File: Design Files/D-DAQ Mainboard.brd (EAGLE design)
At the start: 99.8 x 49.9 mm, 121 parts, among them Y1 XTC7009, Y2 DS1099

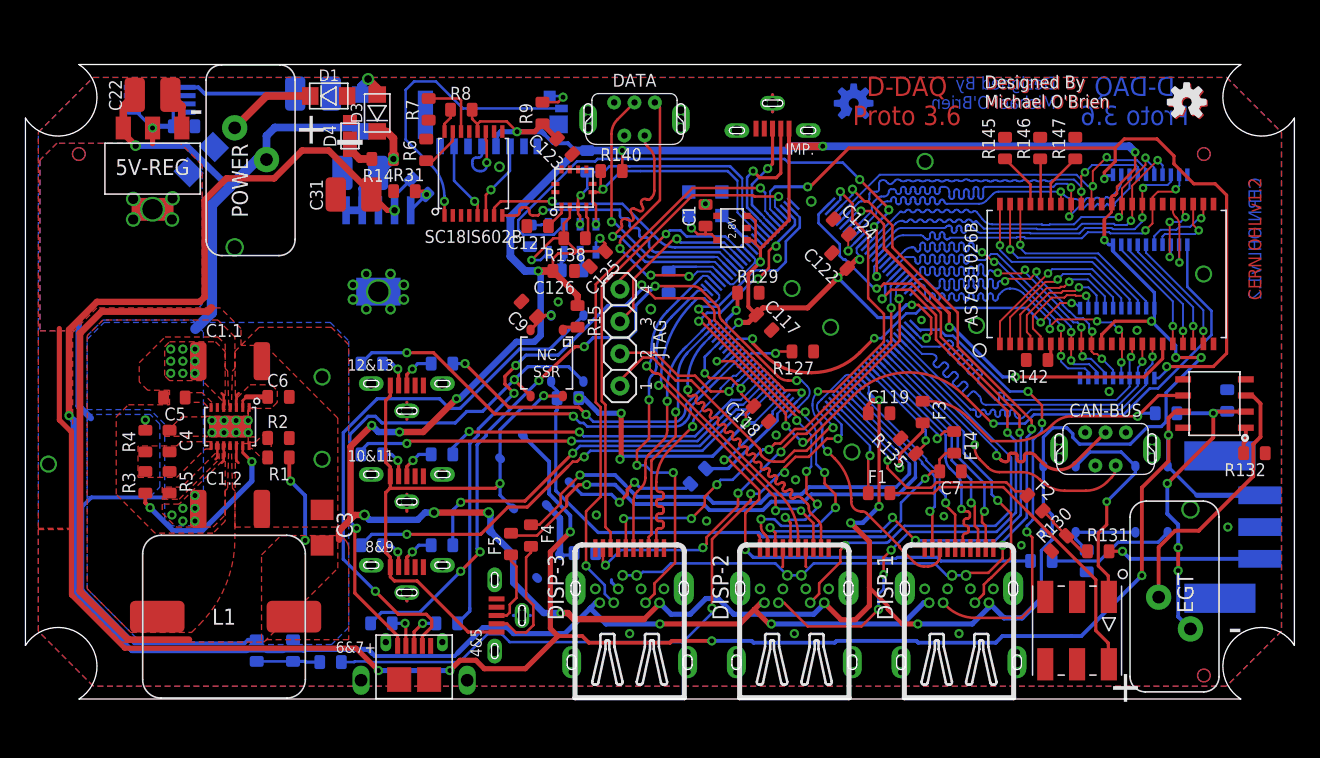
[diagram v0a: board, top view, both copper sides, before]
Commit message: Updating to Proto 4
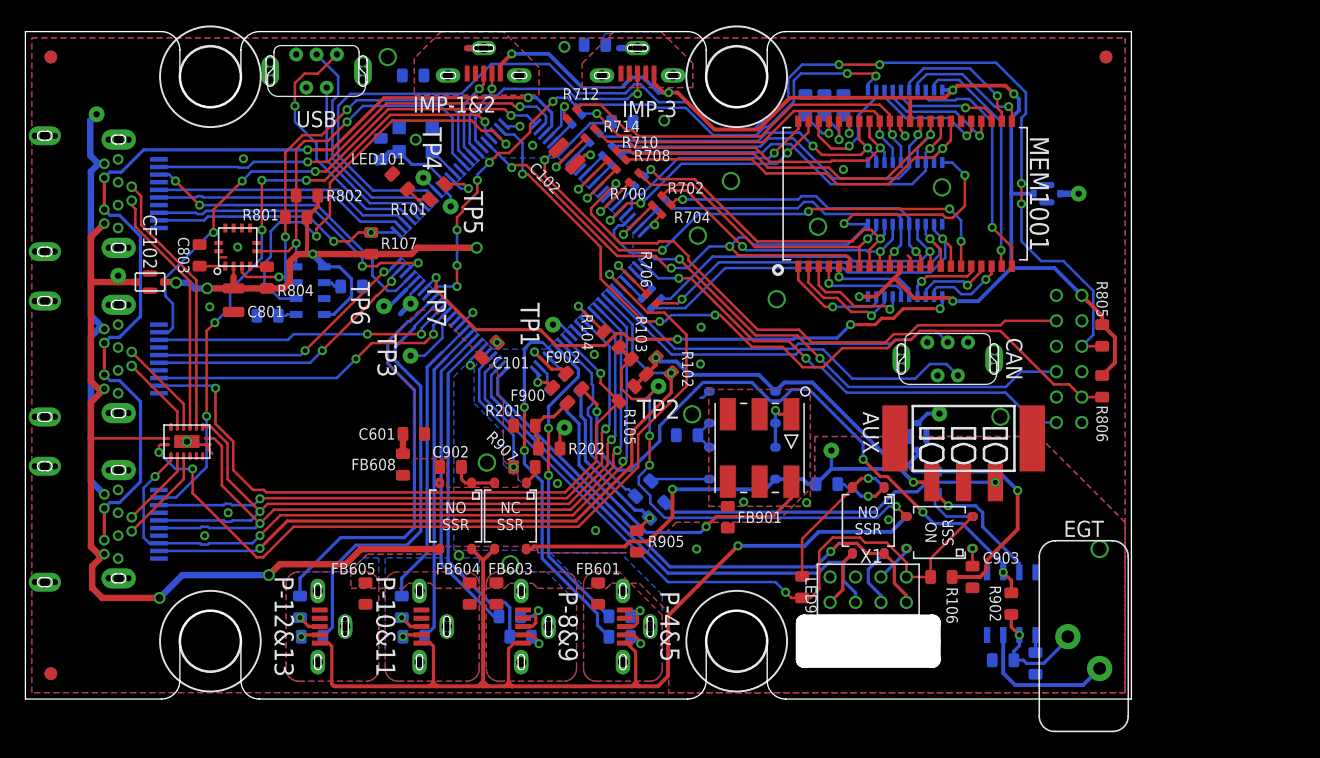
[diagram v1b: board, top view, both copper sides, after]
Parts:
- removed 10&11, 12&13, 4&5, 8&9, IMP.: Micro USB, Parts for D-DAQ:USB-MICRO-B-VERT
- removed 14V-REG: TL1963A-33DCQ, Parts for D-DAQ:SOT-223-6
- removed 2.8V: TC1016-2.8VCTTR, Parts for D-DAQ:SOT-23-5
- removed 3.3V-TOGGLE-1, 3.3V-TOGGLE-2, 3.3V-TOGGLE-3: NO SSR, Parts for D-DAQ:SOP-4-NO
- removed 5V-REG: ZLDO1117-5.0, Parts for D-DAQ:SOT-223-4
- removed 5V-TOGGLE-1, 5V-TOGGLE-2, 5V-TOGGLE-3: NC SSR, Parts for D-DAQ:SOP-4-NC
- removed 6&7+: Micro USB, Parts for D-DAQ:USB-MICRO-AB-FLAT
- removed AS7C31026B: 1 Mbit SRAM, Parts for D-DAQ:TSOP-44
- removed AUX-PRESS: PC-1771101, Parts for D-DAQ:PC-1771101
- removed C1, C6: 10nF, Parts for D-DAQ:SMD-0603
- removed C1.1, C1.2: 22uF, Parts for D-DAQ:SMD-1812-EDGE
- removed C10, C11, C123, C9: 4.7uF, Parts for D-DAQ:SMD-0603
- removed C117, C118, C119, C121, C122, C126, C127, C5, C7, C8: 0.1uF, Parts for D-DAQ:SMD-0603
- removed C124, C125, C2: 22uF, Parts for D-DAQ:SMD-0603
- removed C2.1, C2.2, C22, C31: 10uF, Parts for D-DAQ:SMD-1210
- removed C21: 4.7uF, Parts for D-DAQ:SMD-1206
- removed C3: 47uF, Parts for D-DAQ:SMD-1206
- removed C4: 1uF, Parts for D-DAQ:SMD-0603
- removed CAN-BUS, DATA: UE25BE5510H, Parts for D-DAQ:USB-MINI-B-VERT
- removed D1: S07D-GS08, Parts for D-DAQ:DO-219AB-2
- removed D2, D3: PMEG2010ER, Parts for D-DAQ:DO-219AB-2
- removed D4: TFZGTR20B, Parts for D-DAQ:TUMD2
- removed EGT-AMP: MAX4239, Parts for D-DAQ:SOT-8
- removed F0, F1, F10, F11, F12, F13, F14, F2, F3, F4, F5, F6, F7, F8, F9: 470, Parts for D-DAQ:SMD-0603
- removed JTAG: HEADER-X4, Parts for D-DAQ:HEADER-X4
- removed L1: 7.6uH, Parts for D-DAQ:7443551XXX
- removed LATCH-HIGH, LATCH-LOW: Octal D-Latch, Parts for D-DAQ:TSSOP-20
- removed MAIN-SMPS: MP2209, Parts for D-DAQ:QFN-14
- removed MICRO-SD: 47579-0001, Parts for D-DAQ:SCHA4B0400
- removed MMA8652FC: Accelerometer, Parts for D-DAQ:QFN-12
- removed MPL3115A101: Baro & Temp, Parts for D-DAQ:LGA-8
- removed NBPLANN100PAUNV: Boost, Parts for D-DAQ:LEADLESS-SMT
- removed PIC32MX: 795F512L-80V/PT, Parts for D-DAQ:TQFP-100-12X12
- removed POWER: 1702610, Parts for D-DAQ:PC-1702610
- removed R1: 499k, Parts for D-DAQ:SMD-0603
- removed R10, R12, R127, R129, R130, R132, R135, R138, R139, R142, R145, R146, R147, R6, R7, R8, R9: 10k, Parts for D-DAQ:SMD-0603
- removed R11, R136, R140, R141: 1.4k, Parts for D-DAQ:SMD-0603
- removed R131: 255, Parts for D-DAQ:SMD-0603
- removed R133, R3, R5: 100k, Parts for D-DAQ:SMD-0603
- removed R14: 33.2, Parts for D-DAQ:SMD-0603
- removed R15, R20, R21: 100, Parts for D-DAQ:SMD-0603
- removed R2: 158k, Parts for D-DAQ:SMD-0603
- removed R31: 3.01k, Parts for D-DAQ:SMD-0603
- removed R32: 30.9k, Parts for D-DAQ:SMD-0603
- removed R4: 10, Parts for D-DAQ:SMD-0603
- removed SC18IS602B: I2C to SPI, Parts for D-DAQ:TSSOP-16
- removed U$6, U$7: (no value), Parts for D-DAQ:OSHW-LOGO-S
- removed Y1: XTC7009, Parts for D-DAQ:3.2X2.5MM
- removed Y2: DS1099, Parts for D-DAQ:SOIC-8
- added 12V, 14V, 3.3V, 3.3V-2, 3.3V-3, 5V, TP1, TP2, TP3, TP4, TP5, TP6, TP7: TP-0463, Parts for D-DAQ:TP-REC
- added AUX: PC-3-1771101, Parts for D-DAQ:PC-1771101
- added BFID-1, BFID-2, BFID-3, TFID-1, TFID-2, TFID-3: (no value), Parts for D-DAQ:1MM-FIDUCIAL
- added C101, C601, C802, C803: 0.1uF, Parts for D-DAQ:SMD-0603
- added C102, C801: 10uF, Parts for D-DAQ:SMD-0805
- added C103: 10nF, Parts for D-DAQ:SMD-0603
- added C901, C902, C903: 4.7uF, Parts for D-DAQ:SMD-0603
- added CAN, USB: UE25BE5510H, Parts for D-DAQ:USB-MINI-B-VERT
- added CF101, CF102, CF103: (no value), Parts for D-DAQ:NFM21PS
- added F900, F901, F902, F903, F904, F905, F908, F909, F910, F911, F912, F913, FB601, FB603, FB604, FB605, FB606, FB607, FB608, FB901, R104: 470, Parts for D-DAQ:SMD-0603
- added HOLE-BL, HOLE-BR, HOLE-ML, HOLE-MR: (no value), Parts for D-DAQ:3.2-GRMT
- added IMP-1&2, IMP-3, P-10&11, P-12&13, P-4&5, P-8&9: Micro USB, Parts for D-DAQ:USB-MICRO-B-VERT
- added K1001, K1003, K1005: NC SSR, Parts for D-DAQ:SOP-4-NC
- added K1002, K1004, K1006, K1007, K1008: NO SSR, Parts for D-DAQ:SOP-4-NO
- added LED101: Yellow, Parts for D-DAQ:SMD-0603
- added LED901: Red, Parts for D-DAQ:SMD-0603
- added MEM1001: IS61WV25616ALL, Parts for D-DAQ:TSOP-44
- added OSHW-BOT, OSHW-TOP: (no value), Parts for D-DAQ:OSHW-LOGO-L
- added R101, R102, R103, R105, R106, R107, R202, R716, R717, R718, R719, R803, R804, R805, R806, R903, R905: 10k, Parts for D-DAQ:SMD-0603
- added R201, R801, R802, R901: 1.4k, Parts for D-DAQ:SMD-0603
- added R700, R701, R702, R703, R704, R705, R706, R707, R708, R709, R710, R711, R712, R713, R714, R715: 140, Parts for D-DAQ:SMD-0402
- added R902: 100k, Parts for D-DAQ:SMD-0603
- added R904: 255, Parts for D-DAQ:SMD-0603
- added R906, R907, R908, R909: 100, Parts for D-DAQ:SMD-0603
- added U1001: 795F512L-80V/PT, Parts for D-DAQ:TQFP-100-14X14
- added U1002, U1003: Octal D-Latch, Parts for D-DAQ:TSSOP-20
- added U1004: Baro & Temp, Parts for D-DAQ:LGA-8
- added U1005: Boost, Parts for D-DAQ:LEADLESS-SMT
- added U1006: Accelerometer, Parts for D-DAQ:QFN-12
- added U1007: MAX4239, Parts for D-DAQ:SOT-8
- added U1008: NXP-74HC165, Parts for D-DAQ:DHVQFN16
- added X1: (no value), Parts for D-DAQ:MOLEX-87760-0816
- added X3: MOLEX-87760-1216", Parts for D-DAQ:MOLEX-87760-1216
- added Y1001: XTC7009, Parts for D-DAQ:3.2X2.5MM
- EGT: value 1702610 -> (none)
- moved DISP-1 77.1 mm to (4.25, 39.8), flipped to the bottom, turned to 90 degrees
- moved DISP-2 60.1 mm to (4.25, 26.8), flipped to the bottom, turned to 90 degrees
- moved DISP-3 44.0 mm to (4.25, 13.8), flipped to the bottom, turned to 90 degrees
- moved EGT 7.79 mm to (83.2, 3.65)
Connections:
- removed net 100-PSI-SENSOR-RES: 5V-TOGGLE-2.1, R20.2
- removed net 12V-BS: C5.1, MAIN-SMPS.7
- removed net 12V-ENABLE: MAIN-SMPS.13, R3.1
- removed net 12V-FB: MAIN-SMPS.P14, R1.2, R2.1
- removed net 12V-OK: MAIN-SMPS.9, R5.2
- removed net 12V-SS: C6.1, MAIN-SMPS.2
- removed net 12V-SW: C5.2, L1.P$1, MAIN-SMPS.11, MAIN-SMPS.4
- removed net 12V-VCC: C4.2, MAIN-SMPS.8, R3.2, R4.1, R5.1
- removed net 14V-12V-DIVIDER: F0.2, R10.2, R11.2
- removed net 14V-ADJ: 14V-REG.ADJ, R31.2, R32.1
- removed net 14V-INPUT: 14V-REG.SHDN, 14V-REG.VIN, C2.2.1, D3.P$2, R14.1
- removed net 3.3-&-5V-TOGGLE1: PIC32MX.28, R21.1
- removed net 3.3-&-5V-TOGGLE2: PIC32MX.29, R20.1
- removed net 3.3V-RAIL: 2.8V.1, 2.8V.3, 3.3V-TOGGLE-1.3, 3.3V-TOGGLE-2.3, AS7C31026B.11, AS7C31026B.33, C117.1, C118.2, C119.1, C122.1, C123.2, C125.1, C126.2, C2.2, C3.2, DISP-1.4, DISP-2.4, DISP-3.4, IMP..1, L1.P$2, LATCH-HIGH.20, LATCH-LOW.20, MICRO-SD.4, MMA8652FC.2, MPL3115A101.1, MPL3115A101.4, PIC32MX.16, PIC32MX.2, PIC32MX.30, PIC32MX.37, PIC32MX.46, PIC32MX.55, PIC32MX.62, PIC32MX.86, R1.1, R12.1, R138.2, R140.2, R141.1, R15.1, R8.2, R9.1, SC18IS602B.12
- removed net 5V-ADJ: 5V-REG.ADJ, C22.2
- removed net 6&7-PIN1: 3.3V-TOGGLE-3.3, 5V-TOGGLE-3.3, 6&7+.1
- removed net A0-PD: R7.2, SC18IS602B.14
- removed net A1-PD: R6.1, SC18IS602B.15
- removed net A2-PU: R8.1, SC18IS602B.16
- removed net ADD-0: AS7C31026B.5, LATCH-LOW.12
- removed net ADD-1: AS7C31026B.4, LATCH-LOW.13
- removed net ADD-10: AS7C31026B.25, LATCH-HIGH.14
- removed net ADD-11: AS7C31026B.24, LATCH-HIGH.15
- removed net ADD-12: AS7C31026B.21, LATCH-HIGH.16
- removed net ADD-13: AS7C31026B.20, LATCH-HIGH.17
- removed net ADD-14: AS7C31026B.19, LATCH-HIGH.18
- removed net ADD-15: AS7C31026B.18, LATCH-HIGH.19
- removed net ADD-2: AS7C31026B.3, LATCH-LOW.14
- removed net ADD-3: AS7C31026B.2, LATCH-LOW.15
- removed net ADD-4: AS7C31026B.1, LATCH-LOW.16
- removed net ADD-5: AS7C31026B.44, LATCH-LOW.17
- removed net ADD-6: AS7C31026B.43, LATCH-LOW.18
- removed net ADD-7: AS7C31026B.42, LATCH-LOW.19
- removed net ADD-8: AS7C31026B.27, LATCH-HIGH.12
- removed net ADD-9: AS7C31026B.26, LATCH-HIGH.13
- removed net AN2-OIL-PESS: F2.1, PIC32MX.23
- removed net AN3-EGT: F3.2, PIC32MX.22
- removed net AN6: 6&7+.2, F6.1
- removed net AN7: 6&7+.3, F7.2
- removed net AUTO-DETECT: 5V-TOGGLE-1.1, R21.2
- removed net BARO-INT2: MPL3115A101.5, R139.1
- removed net CAN-BUS1: CAN-BUS.2, PIC32MX.8
- removed net CAN-BUS2: CAN-BUS.3, PIC32MX.7
- removed net CARD-DETECT: MICRO-SD.G3, SC18IS602B.1
- removed net CE: AS7C31026B.6, R142.1
- removed net CHARG-CAPS: C2.1.1, Y2.1
- removed net CP-PUMP: C2.1.2, D2.P$2, D3.P$1
- removed net CPS-INPUT: IMP..2, PIC32MX.68
- removed net CRYSTAL-OUT: PIC32MX.63
- removed net DISP-1_HPD: DISP-1.6, PIC32MX.9
- removed net DISP-HPD2: DISP-2.6, PIC32MX.6
- removed net DISP-HPD3: DISP-3.6, PIC32MX.51
- removed net EGT-SHTDWN: EGT-AMP.1, R132.2
- removed net GND: 10&11.5, 10&11.T0, 10&11.T1, 10&11.T2, 12&13.5, 12&13.T0, 12&13.T1, 12&13.T2, 14V-REG.GND, 14V-REG.TAB, 2.8V.2, 3.3V-TOGGLE-1.2, 3.3V-TOGGLE-2.2, 4&5.5, 4&5.T0, 4&5.T1, 4&5.T2, 6&7+.5, 6&7+.B1, 6&7+.B2, 6&7+.F1, 6&7+.F2, 8&9.5, 8&9.T0, 8&9.T1, 8&9.T2, AS7C31026B.12, AS7C31026B.34, AUX-PRESS.P2, AUX-PRESS.T0, AUX-PRESS.T1, C1.1.2, C1.2, C1.2.2, C10.1, C11.1, C117.2, C118.1, C119.2, C121.2, C122.2, C123.1, C124.1, C125.2, C126.1, C127.1, C2.1, C2.2.2, C21.2, C3.1, C31.1, C4.1, C6.2, C7.1, C8.2, C9.2, CAN-BUS.5, CAN-BUS.P$1, CAN-BUS.P$2, CAN-BUS.P$3, CAN-BUS.P$4, CAN-BUS.T0, CAN-BUS.T1, D1.P$1, D4.P$1, DATA.5, DATA.P$1, DATA.P$2, DATA.P$3, DATA.P$4, DATA.T0, DATA.T1, DISP-1.1, DISP-1.13, DISP-1.14, DISP-1.19, DISP-1.7, DISP-1.8, DISP-1.BL, DISP-1.BR, DISP-1.FL, DISP-1.FR, DISP-2.1, DISP-2.13, DISP-2.14, DISP-2.19, DISP-2.7, DISP-2.8, DISP-2.BL, DISP-2.BR, DISP-2.FL, DISP-2.FR, DISP-3.1, DISP-3.13, DISP-3.14, DISP-3.19, DISP-3.7, DISP-3.8, DISP-3.BL, DISP-3.BR, DISP-3.FL, DISP-3.FR, EGT-AMP.4, IMP..5, IMP..T0, IMP..T1, IMP..T2, LATCH-HIGH.10, LATCH-LOW.10, MAIN-SMPS.1, MAIN-SMPS.12, MAIN-SMPS.3, MAIN-SMPS.P$15, MICRO-SD.6, MICRO-SD.G1, MICRO-SD.G2, MMA8652FC.6, MMA8652FC.7, MPL3115A101.3, NBPLANN100PAUNV.4, PIC32MX.15, PIC32MX.31, PIC32MX.36, PIC32MX.45, PIC32MX.65, PIC32MX.75, R11.1, R127.1, R129.2, R130.1, R132.1, R135.2, R136.2, R139.2, R142.2, R145.2, R146.2, R147.2, R2.2, R31.1, R6.2, R7.1, SC18IS602B.4, Y1.P$1, Y1.P$2, Y2.4, Y2.6
- removed net HB: AS7C31026B.40, R146.1
- removed net I2C-INT-BUS-PIN1: MPL3115A101.6, PIC32MX.91
- removed net I2C-INT-BUS-PIN2: PIC32MX.92
- removed net I2C-PIN1: MMA8652FC.5, MPL3115A101.8, PIC32MX.66, R140.1
- removed net I2C-PIN2: MMA8652FC.3, MPL3115A101.7, PIC32MX.67, R141.2
- removed net I2C-SD-PIN1: PIC32MX.58, SC18IS602B.8
- removed net I2C-SD-PIN2: PIC32MX.59, SC18IS602B.7
- removed net ICSP-MCLR: 3.3V-TOGGLE-3.4, C7.2, F14.2, R12.2
- removed net ICSP-TRIP: 3.3V-TOGGLE-3.2, 6&7+.4
- removed net ICSP-TRIP-PWR: 5V-TOGGLE-3.1, R15.2
- removed net LB: AS7C31026B.39, R147.1
- removed net LNS-INPUT: IMP..3, PIC32MX.69
- removed net N$5: C121.1, MMA8652FC.1
- removed net OE: AS7C31026B.41, R145.1
- removed net OSC-PWR: 2.8V.5, C1.1, Y1.P$4
- removed net OSC-SIG: PIC32MX.64, Y1.P$3
- removed net PMA-CS2: DISP-3.16, PIC32MX.70
- removed net PMA-HL: LATCH-HIGH.11, PIC32MX.43
- removed net PMD-READ: PIC32MX.82
- removed net PWM1: DISP-3.15, PIC32MX.72
- removed net PWM2: DISP-2.15, PIC32MX.76
- removed net PWM3: DISP-1.15, PIC32MX.77
- removed net PWM4: DISP-1.10, DISP-1.12, DISP-2.10, DISP-2.12, DISP-3.10, DISP-3.12, PIC32MX.78
- removed net PWR-GND: D1.P$2, POWER.R
- removed net SD-MISO: MICRO-SD.7, SC18IS602B.5
- removed net SD-MOSI: MICRO-SD.3, SC18IS602B.6
- removed net SD-PULL-DOWN: MICRO-SD.G4, R9.2
- removed net SENSOR_PAIR_AN10: F10.2, PIC32MX.34
- removed net SENSOR_PAIR_AN11: F11.1, PIC32MX.35
- removed net SENSOR_PAIR_AN12: F12.2, PIC32MX.41
- removed net SENSOR_PAIR_AN13: F13.1, PIC32MX.42
- removed net SENSOR_PAIR_AN4: F4.1, PIC32MX.21
- removed net SENSOR_PAIR_AN5: F5.2, PIC32MX.20
- removed net SENSOR_PAIR_AN6: F6.2, PIC32MX.26
- removed net SENSOR_PAIR_AN7: F7.1, PIC32MX.27
- removed net SENSOR_PAIR_AN8: F8.2, PIC32MX.32
- removed net SENSOR_PAIR_AN9: F9.1, PIC32MX.33
- removed net SHUNT: D4.P$2, R14.2
- removed net SPI2-DATA: DISP-1.9, PIC32MX.12
- removed net SPI2-SS: PIC32MX.14, R135.1
- removed net SPI3-DATA: DISP-2.9, PIC32MX.53
- removed net SPI3-SS: PIC32MX.47, R129.1
- removed net SPI4-CLK: DISP-3.3, PIC32MX.39
- removed net SPI4-DATA: DISP-3.9, PIC32MX.50
- removed net SPI4-SS: PIC32MX.40, R127.2
- removed net USB-PIN1: DATA.1, PIC32MX.54
- removed net USB-PIN2: DATA.2, PIC32MX.56
- removed net USB-PIN3: DATA.3, PIC32MX.57
- new net 3.3V-RAIL-1: 3.3V-2.TP, CF101.1
- new net 3.3V-RAIL-2: 3.3V.TP, CF102.1, DISP-1.18, DISP-2.18, DISP-3.18, K1004.3, U1008.VCC
- new net 3.3V-RAIL-3: 3.3V-3.TP, CF103.1
- new net 6&7-PIN-1: K1005.3, K1006.4, X1.6
- new net ACCEL-BYP: C803.1, U1006.1
- new net ADT-1: K1001.1, R906.2
- new net ADT-2: K1003.1, R907.2
- new net ADT-3: K1005.1, R908.2
- new net ADT-4: K1007.1, K1008.1, R909.2
- new net AGND: AUX.P2, AUX.T0, AUX.T1, C101.2, C601.1, C903.2, CF101.2@1, CF101.2@2, FB601.2, FB603.2, FB604.2, FB605.2, FB901.2, R901.1, R903.2, R905.2, U1001.31, U1007.4, X1.8
- new net ALT-INT: U1001.73, U1004.6
- new net AN2-EGT: F902.2, U1001.23
- new net AN3-AUX-PRESS: F903.2, U1001.22
- new net BARO-INT: R803.2, U1004.5
- new net BOOST-GND: FB901.1, U1005.4
- new net BOOST-V-TOGGLE: R906.1, U1001.19
- new net CAN-BUS-1: CAN.2, U1001.8
- new net CAN-BUS-2: CAN.3, U1001.7
- new net CLEAN-3.3V-1: CF101.3, K1002.3, R102.1, R103.1, R105.1, R106.1, R908.1
- new net CLEAN-3.3V-2: C101.1, C103.1, C801.1, CF102.3, R107.2, R801.1, R802.1, R804.1, TP6.TP, U1001.16, U1001.2, U1001.30, U1001.37, U1001.46, U1001.55, U1001.62, U1001.86, U1004.1, U1004.4, U1006.2, Y1001.P$4
- new net CLEAN-3.3V-3: CF103.3, IMP-1&2.1, IMP-3.1, MEM1001.11, MEM1001.33, R805.1, R806.1, U1002.20, U1003.20, X3.7
- new net DGND: C102.2, C103.2, C801.2, C802.1, C803.2, C901.1, C902.1, CAN.5, CAN.P$1, CAN.P$2, CAN.P$3, CAN.P$4, CAN.T0, CAN.T1, CF102.2@1, CF102.2@2, CF103.2@1, CF103.2@2, DISP-1.1, DISP-1.13, DISP-1.14, DISP-1.19, DISP-1.7, DISP-1.8, DISP-1.BL, DISP-1.BR, DISP-1.FL, DISP-1.FR, DISP-2.1, DISP-2.13, DISP-2.14, DISP-2.19, DISP-2.7, DISP-2.8, DISP-2.BL, DISP-2.BR, DISP-2.FL, DISP-2.FR, DISP-3.1, DISP-3.13, DISP-3.14, DISP-3.19, DISP-3.7, DISP-3.8, DISP-3.BL, DISP-3.BR, DISP-3.FL, DISP-3.FR, FB606.2, FB607.2, FB608.1, K1002.2, K1004.2, LED101.2, MEM1001.12, MEM1001.34, R201.1, R716.2, R717.2, R718.2, R719.2, R803.1, TP7.TP, U1001.15, U1001.36, U1001.45, U1001.65, U1001.75, U1002.10, U1003.10, U1004.3, U1006.6, U1006.7, U1008.-CE, U1008.GND, U1008.GND2, USB.5, USB.P$1, USB.P$2, USB.P$3, USB.P$4, USB.T0, USB.T1, X3.10, X3.12, X3.2, X3.4, X3.6, X3.8, Y1001.P$1, Y1001.P$2
- new net DISP1-HPD: DISP-1.17, R107.1, U1001.51
- new net DISP1-RS: DISP-1.5, U1001.47
- new net DISP2-HPD: DISP-2.17, R105.2, U1001.18
- new net DISP3-HPD: DISP-3.17, R102.2, U1001.9
- new net EGT-SHDN: R903.1, U1007.1
- new net GND-FILTER: C601.2, FB608.2
- new net HB-PD: MEM1001.40, R717.1
- new net I2C-CLK: R802.2, U1001.66, U1004.8, U1006.5
- new net I2C-DATA: R801.2, U1001.67, U1004.7, U1006.3
- new net ICSP-DETECT: K1006.2, LED901.2, R106.2, U1001.28, X1.5
- new net ICSP-LED: K1007.2, K1008.2, LED901.1
- new net IMP-1: IMP-1&2.3, U1001.68
- new net IMP-2: IMP-1&2.2, U1001.69
- new net IMP-3: IMP-3.3, U1001.70
- new net INPUT-V-SENSE: F900.1, R201.2, R202.2
- new net LB-PD: MEM1001.39, R716.1
- new net LOAD-AN6: K1007.3, X1.1
- new net LOAD-AN7: K1008.3, X1.3
- new net N$58: U1001.58
- new net NC$1: X1.7
- new net OE-PD: MEM1001.41, R718.1
- new net OSCI: U1001.64, Y1001.P$3
- new net PMA-LH: U1001.43, U1003.11
- new net PMD-0: MEM1001.7, R700.2, U1002.2
- new net PMD-1: MEM1001.8, R701.2, U1002.3
- new net PMD-10: MEM1001.31, R710.2, U1003.4
- new net PMD-11: MEM1001.32, R711.2, U1003.5
- new net PMD-12: MEM1001.35, R712.2, U1003.6
- new net PMD-13: MEM1001.36, R713.2, U1003.7
- new net PMD-15: MEM1001.38, R715.2, U1003.9
- new net PMD-2: MEM1001.9, R702.2, U1002.4
- new net PMD-3: MEM1001.10, R703.2, U1002.5
- new net PMD-4: MEM1001.13, R704.2, U1002.6
- new net PMD-5: MEM1001.14, R705.2, U1002.7
- new net PMD-6: MEM1001.15, R706.2, U1002.8
- new net PMD-7: MEM1001.16, R707.2, U1002.9
- new net PMD-8: MEM1001.29, R708.2, U1003.2
- new net PMD-9: MEM1001.30, R709.2, U1003.3
- new net PMD14: R714.1, U1001.83
- new net PMP-READ: R719.1, U1001.82
- new net PWM-BL: DISP-1.16, DISP-1.6, DISP-2.16, DISP-2.6, DISP-3.16, DISP-3.6, U1001.78
- new net PWM1-WARN: DISP-1.3, U1001.77
- new net PWM2-WARN: DISP-2.3, U1001.76
- new net PWM3-WARN: DISP-3.3, U1001.72
- new net SD-CARD-DETECT: R805.2, U1001.59, X3.9
- new net SD-SPI-DI: U1001.92, X3.5
- new net SD-SPI-DO: U1001.1, X3.1
- new net SD-WRITE-PROTECT: R806.2, U1001.74, X3.11
- new net SENSOR-AN10: F910.2, U1001.34
- new net SENSOR-AN11: F911.2, U1001.35
- new net SENSOR-AN12: F912.2, U1001.41
- new net SENSOR-AN13: F913.2, U1001.42
- new net SENSOR-AN4: F904.1, U1001.21
- new net SENSOR-AN5: F905.1, U1001.20
- new net SENSOR-AN6: K1007.4, U1001.26, X1.4
- new net SENSOR-AN7: K1008.4, U1001.27, X1.2
- new net SENSOR-AN8: F908.2, U1001.32
- new net SENSOR-AN9: F909.2, U1001.33
- new net SGND-1: FB601.1, P-4&5.5, P-4&5.T0, P-4&5.T1, P-4&5.T2
- new net SGND-3: FB603.1, P-8&9.5, P-8&9.T0, P-8&9.T1, P-8&9.T2
- new net SGND-4: FB604.1, P-10&11.5, P-10&11.T0, P-10&11.T1, P-10&11.T2
- new net SGND-5: FB605.1, P-12&13.5, P-12&13.T0, P-12&13.T1, P-12&13.T2
- new net SGND-6: FB606.1, IMP-1&2.5, IMP-1&2.T0, IMP-1&2.T1, IMP-1&2.T2
- new net SGND-7: FB607.1, IMP-3.5, IMP-3.T0, IMP-3.T1, IMP-3.T2
- new net SHIFT-CS-LINE: U1001.6, U1008.-PL
- new net SOFT-PMP-CS2: U1001.91
- new net SPI1-CLK: DISP-1.15, U1001.48
- new net SPI1-DO: DISP-1.9, U1001.53
- new net SPI2-DO: DISP-2.9, U1001.50
- new net SPI3-DO: DISP-3.9, U1001.12, U1008.DS
- new net SRAM-0: MEM1001.1, U1002.19
- new net SRAM-1: MEM1001.2, U1002.18
- new net SRAM-10: MEM1001.23, U1003.17
- new net SRAM-11: MEM1001.24, U1003.16
- new net SRAM-12: MEM1001.25, U1003.15
- new net SRAM-13: MEM1001.26, U1003.14
- new net SRAM-14: MEM1001.27, U1003.13
- new net SRAM-15: MEM1001.42, U1003.12
- new net SRAM-16: MEM1001.43, U1001.95
- new net SRAM-17: MEM1001.44, U1001.96
- new net SRAM-2: MEM1001.3, U1002.17
- new net SRAM-3: MEM1001.4, U1002.16
- new net SRAM-4: MEM1001.5, U1002.15
- new net SRAM-5: MEM1001.18, U1002.14
- new net SRAM-6: MEM1001.19, U1002.13
- new net SRAM-7: MEM1001.20, U1002.12
- new net SRAM-8: MEM1001.21, U1003.19
- new net SRAM-9: MEM1001.22, U1003.18
- new net SRST-MCLR: K1006.3, R103.2, R104.1, TP2.TP
- new net STATUS: R101.1, U1001.63
- new net STATUS-LED: LED101.1, R101.2
- new net USB-PIN-1: U1001.54, USB.1
- new net USB-PIN-2: U1001.56, USB.2
- new net USB-PIN-3: U1001.57, USB.3
- new net USB-V-TOGGLE: R907.1, U1001.29
- net 12V-INPUT: now also 12V.TP, R202.1; no longer 5V-REG.VIN, C1.1.1, C1.2.1, C22.1, D2.P$1, MAIN-SMPS.10, MAIN-SMPS.5, POWER.L, R10.1
- net 14V-RAIL: now also 14V.TP, DISP-1.4, DISP-2.4, DISP-3.4; no longer 14V-REG.VOUT, C31.2, DISP-1.18, DISP-2.18, DISP-3.18, R32.2
- net 5V-RAIL: now also 5V.TP, AUX.P1, K1001.4, K1003.4, R909.1, U1007.7; no longer 5V-REG.VOUT, 5V-REG.VOUT-1, 5V-TOGGLE-1.4, 5V-TOGGLE-2.4, AUX-PRESS.P1, C21.1, C8.1, EGT-AMP.7, R4.2, Y2.3, Y2.5
- net ACCEL-EN: now also R804.2, U1006.4; no longer MMA8652FC.4, R138.1
- net AN0-VOLT: now also F900.2, U1001.25; no longer F0.1, PIC32MX.25
- net AN1-BOOST: now also F901.2, U1001.24; no longer F1.1, PIC32MX.24
- net AN10: now also F910.1, P-10&11.2; no longer 10&11.2, F10.1
- net AN11: now also F911.1, P-10&11.3; no longer 10&11.3, F11.2
- net AN12: now also F912.1, P-12&13.2; no longer 12&13.2, F12.1
- net AN13: now also F913.1, P-12&13.3; no longer 12&13.3, F13.2
- net AN4: now also F904.2, P-4&5.2; no longer 4&5.2, F4.2
- net AN5: now also F905.2, P-4&5.3; no longer 4&5.3, F5.1
- net AN8: now also F908.1, P-8&9.2; no longer 8&9.2, F8.1
- net AN9: now also F909.1, P-8&9.3; no longer 8&9.3, F9.2
- net AUX-OUT: now also F903.1, R904.2, R905.1; no longer F2.2, R130.2, R131.1
- net BOOST-OUT: now also F901.1, U1005.6; no longer F1.2, NBPLANN100PAUNV.6
- net BOOST-PWR: now also K1001.3, K1002.4, U1005.1; no longer 3.3V-TOGGLE-2.4, 5V-TOGGLE-2.3, NBPLANN100PAUNV.1
- net BOOST-SSR: now also C901.2, K1001.2, K1002.1; no longer 3.3V-TOGGLE-2.1, 5V-TOGGLE-2.2, C11.2
- net DISP1-B1: now also DISP-1.11, U1001.52; no longer DISP-1.5, PIC32MX.11
- net DISP1-B2: now also DISP-1.12, U1008.D1; no longer DISP-1.11, PIC32MX.18
- net DISP1-B3: now also DISP-1.10, U1008.D0; no longer DISP-1.17, PIC32MX.19
- net DISP2-B1: now also DISP-2.11, U1001.49; no longer DISP-2.5, PIC32MX.52
- net DISP2-B2: now also DISP-2.12, U1008.D3; no longer DISP-2.11, PIC32MX.73
- net DISP2-B3: now also DISP-2.10, U1008.D2; no longer DISP-2.17, PIC32MX.74
- net DISP2-RS: now also DISP-2.5, U1001.40; no longer DISP-2.16, PIC32MX.95
- net DISP3-B1: now also DISP-3.11, U1001.11, U1008.Q7; no longer DISP-3.5, PIC32MX.49
- net DISP3-B2: now also DISP-3.12, U1008.D5; no longer DISP-3.11, PIC32MX.96
- net DISP3-B3: now also DISP-3.10, U1008.D4; no longer DISP-3.17, PIC32MX.97
- net DISP3-RS: now also DISP-3.5, U1001.14; no longer DISP-1.16, PIC32MX.1
- net EGT-NEG-IN: now also EGT.L, R901.2, R902.1, U1007.2; no longer EGT-AMP.2, EGT.R, R133.1, R136.1
- net EGT-OUT: now also F902.1, R902.2, U1007.6; no longer EGT-AMP.6, F3.1, R133.2
- net EGT-POS-IN: now also EGT.R, U1007.3; no longer EGT-AMP.3, EGT.L
- net ICSP-SSR: now also C903.1, K1005.2, K1006.1; no longer 3.3V-TOGGLE-3.1, 5V-TOGGLE-3.2, C9.1
- net JTAG-PIN-1: now also TP1.TP, U1001.17; no longer JTAG.1, PIC32MX.17
- net JTAG-PIN-2: now also TP3.TP, U1001.38; no longer JTAG.2, PIC32MX.38
- net JTAG-PIN-3: now also TP4.TP, U1001.60; no longer JTAG.3, PIC32MX.60
- net JTAG-PIN-4: now also TP5.TP, U1001.61; no longer JTAG.4, PIC32MX.61
- net MCLR: now also R104.2, U1001.13; no longer F14.1, PIC32MX.13
- net MPL-BYP-CAP: now also C802.2, U1004.2; no longer C127.2, MPL3115A101.2
- net OIL-PRESS-OUT: now also AUX.P3, R904.1; no longer AUX-PRESS.P3, R131.2
- net P$1: now also CAN.1; no longer CAN-BUS.1
- net PMA-LL: now also U1001.44, U1002.11; no longer LATCH-LOW.11, PIC32MX.44
- net PMD-14: now also MEM1001.37, R714.2, U1003.8; no longer AS7C31026B.37, LATCH-HIGH.3, PIC32MX.83
- net PMD0: now also R700.1, U1001.93; no longer AS7C31026B.7, LATCH-LOW.9, PIC32MX.93
- net PMD1: now also R701.1, U1001.94; no longer AS7C31026B.8, LATCH-LOW.8, PIC32MX.94
- net PMD10: now also R710.1, U1001.88; no longer AS7C31026B.31, LATCH-HIGH.7, PIC32MX.88
- net PMD11: now also R711.1, U1001.87; no longer AS7C31026B.32, LATCH-HIGH.6, PIC32MX.87
- net PMD12: now also R712.1, U1001.79; no longer AS7C31026B.35, LATCH-HIGH.5, PIC32MX.79
- net PMD13: now also R713.1, U1001.80; no longer AS7C31026B.36, LATCH-HIGH.4, PIC32MX.80
- net PMD15: now also R715.1, U1001.84; no longer AS7C31026B.38, LATCH-HIGH.2, PIC32MX.84
- net PMD2: now also R702.1, U1001.98; no longer AS7C31026B.9, LATCH-LOW.7, PIC32MX.98
- net PMD3: now also R703.1, U1001.99; no longer AS7C31026B.10, LATCH-LOW.6, PIC32MX.99
- net PMD4: now also R704.1, U1001.100; no longer AS7C31026B.13, LATCH-LOW.5, PIC32MX.100
- net PMD5: now also R705.1, U1001.3; no longer AS7C31026B.14, LATCH-LOW.4, PIC32MX.3
- net PMD6: now also R706.1, U1001.4; no longer AS7C31026B.15, LATCH-LOW.3, PIC32MX.4
- net PMD7: now also R707.1, U1001.5; no longer AS7C31026B.16, LATCH-LOW.2, PIC32MX.5
- net PMD8: now also R708.1, U1001.90; no longer AS7C31026B.29, LATCH-HIGH.9, PIC32MX.90
- net PMD9: now also R709.1, U1001.89; no longer AS7C31026B.30, LATCH-HIGH.8, PIC32MX.89
- net PMP-CS1: now also MEM1001.6, U1001.71, U1002.1, U1003.1; no longer LATCH-HIGH.1, LATCH-LOW.1, PIC32MX.71
- net PMP-WRITE: now also MEM1001.17, U1001.81; no longer AS7C31026B.17, PIC32MX.81
- net SD-SPI-CLK: now also U1001.97, X3.3; no longer MICRO-SD.5, SC18IS602B.11
- net SPI2-CLK: now also DISP-2.15, U1001.39; no longer DISP-1.3, PIC32MX.10
- net SPI3-CLK: now also DISP-3.15, U1001.10, U1008.CP; no longer DISP-2.3, PIC32MX.48
- net USB-PWR: now also K1003.3, K1004.4, K1005.4, P-10&11.1, P-12&13.1, P-4&5.1, P-8&9.1; no longer 10&11.1, 12&13.1, 3.3V-TOGGLE-1.4, 4&5.1, 5V-TOGGLE-1.3, 5V-TOGGLE-3.4, 8&9.1
- net USB-SSR: now also C902.2, K1003.2, K1004.1; no longer 3.3V-TOGGLE-1.1, 5V-TOGGLE-1.2, C10.2
- net V-CAP: now also C102.1, U1001.85; no longer C124.2, PIC32MX.85
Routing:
- net 3.3V-RAIL: track 380.7 -> 0.00 mm, vias 36 -> 0
- net 5V-RAIL: track 172.3 -> 49.2 mm, vias 13 -> 3
- net 14V-RAIL: track 137.2 -> 32.7 mm, vias 4 -> 0
- net SD-CARD-DETECT: track 0.00 -> 100.3 mm, vias 0 -> 4
- net CLEAN-3.3V-3: track 0.00 -> 97.8 mm, vias 0 -> 6
- net PWM-BL: track 0.00 -> 75.1 mm, vias 0 -> 2
- net 3.3V-RAIL-2: track 0.00 -> 70.6 mm, vias 0 -> 2
- net PWM4: track 70.3 -> 0.00 mm, vias 3 -> 0
- net 12V-INPUT: track 70.9 -> 1.79 mm, vias 16 -> 0
- net SHIFT-CS-LINE: track 0.00 -> 67.5 mm, vias 0 -> 3
- net SD-WRITE-PROTECT: track 0.00 -> 61.8 mm, vias 0 -> 3
- net SPI3-DO: track 0.00 -> 59.0 mm, vias 0 -> 2
- net SENSOR_PAIR_AN6: track 57.8 -> 0.00 mm, vias 6 -> 0
- net PWM2: track 57.5 -> 0.00 mm, vias 5 -> 0
- net DISP3-HPD: track 0.00 -> 57.4 mm, vias 0 -> 2
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- added copper zone on layer 1, net AGND
- added copper zone on layer 16, net AGND
- added copper zone on layer 1, net BOOST-GND
- added copper zone on layer 16, net BOOST-GND
- added copper zone on layer 16, net CLEAN-3.3V-2
- added copper zone on layer 1, net DGND
- added copper zone on layer 16, net DGND
- added copper zone on layer 1, net SGND-1
- added copper zone on layer 16, net SGND-1
- added copper zone on layer 1, net SGND-3
- added copper zone on layer 16, net SGND-3
- added copper zone on layer 1, net SGND-4
- added copper zone on layer 16, net SGND-4
- added copper zone on layer 1, net SGND-5
- added copper zone on layer 16, net SGND-5
- added copper zone on layer 1, net SGND-6
- added copper zone on layer 16, net SGND-6
- added copper zone on layer 1, net SGND-7
- added copper zone on layer 16, net SGND-7
- removed copper zone on layer 1, net 12V-BS
- removed copper zone on layer 1, net 12V-FB
- removed copper zone on layer 1, net 12V-INPUT
- removed copper zone on layer 16, net 12V-INPUT
- removed copper zone on layer 1, net 12V-OK
- removed copper zone on layer 1, net 12V-SW
- removed copper zone on layer 1, net 12V-VCC
- removed copper zone on layer 1, net 3.3V-RAIL
- removed copper zone on layer 1, net 5V-RAIL
- removed copper zone on layer 16, net 5V-RAIL
- removed copper zone on layer 16, net FD-B1
- removed copper zone on layer 16, net FD-B2
- removed copper zone on layer 16, net FD-B3
- removed copper zone on layer 1, net FD-F1
- removed copper zone on layer 1, net FD-F2
- removed copper zone on layer 1, net FD-F3
- removed copper zone on layer 1, net GND
- removed copper zone on layer 16, net GND
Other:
- board size 99.8 x 49.9 mm -> 87 x 52.5 mm
- board text added: "Created By M.O'B"
- board text added: "D-DAQ"
- board text removed: "+"
- board text removed: "-"
- board text removed: "5"
- board text removed: "D-DAQ Proto 3.6"
- board text removed: "Designed By Michael O'Brien"
